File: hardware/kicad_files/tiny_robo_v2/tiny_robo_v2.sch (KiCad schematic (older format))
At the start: 31 parts, among them P1 CONN_01X06, P2 BATT, P3 CONN_01X02, P4 CONNECTOR, P5 CONNECTOR, P6 CONN_01X02, SW1 SPDT, U1 MCP73831, U2 MIC5265, U3 ESP8266-ESP-03, U4 DRV8830, U5 DRV8830

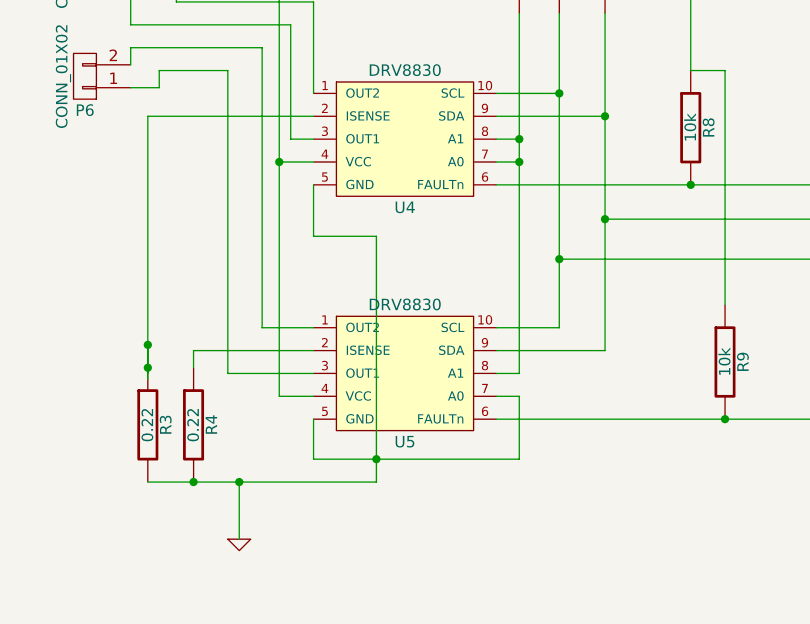
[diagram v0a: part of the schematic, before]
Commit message: syncing home version
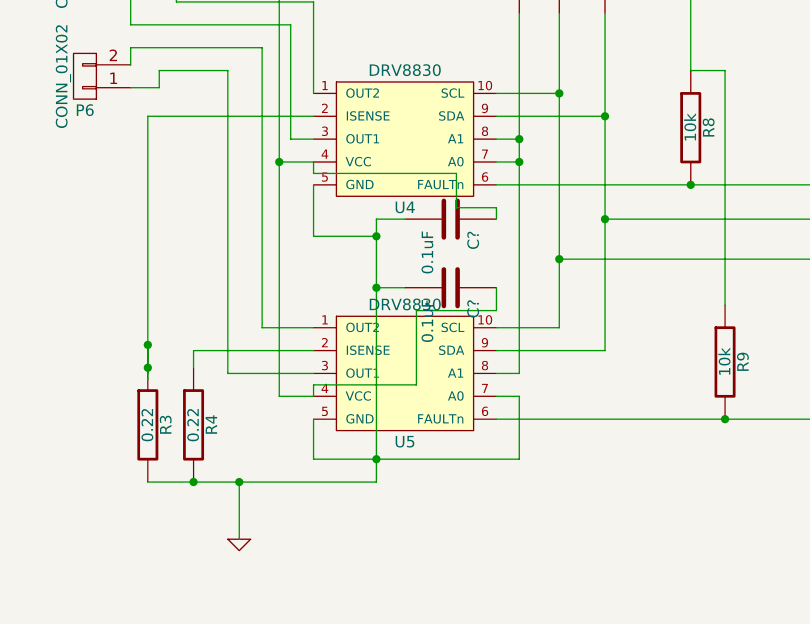
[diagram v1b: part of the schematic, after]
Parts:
- added C? (x2): 0.1uF, Capacitors_SMD:C_0805_HandSoldering, symbol C-RESCUE-tiny_robo_v2
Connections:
- net GND: now also C?.2, C?.2
- net Unreg: now also C?.1, C?.1
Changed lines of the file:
@@
 EESchema Schematic File Version 2
+LIBS:tiny_robo_v2-rescue
 LIBS:power
 LIBS:device
@@
 	5650 1300 6275 1300
 Wire Wire Line
-	8650 5525 8650 6600
+	8650 5450 8650 6600
 Connection ~ 7850 6600
 Connection ~ 9650 3775
@@
 Wire Wire Line
 	2975 4125 2400 4125
+$Comp
+L C-RESCUE-tiny_robo_v2 C?
+U 1 1 57E440DA
+P 8975 5450
+F 0 "C?" H 9025 5550 50  0000 L CNN
+F 1 "0.1uF" H 9025 5350 50  0000 L CNN
+F 2 "Capacitors_SMD:C_0805_HandSoldering" H 8975 5450 60  0001 C CNN
+F 3 "" H 8975 5450 60  0001 C CNN
+	1    8975 5450
+	0    1    1    0
+$EndComp
+$Comp
+L C-RESCUE-tiny_robo_v2 C?
+U 1 1 57E442F8
+P 8975 5750
+F 0 "C?" H 9025 5850 50  0000 L CNN
+F 1 "0.1uF" H 9025 5650 50  0000 L CNN
+F 2 "Capacitors_SMD:C_0805_HandSoldering" H 8975 5750 60  0001 C CNN
+F 3 "" H 8975 5750 60  0001 C CNN
+	1    8975 5750
+	0    1    1    0
+$EndComp
+Wire Wire Line
+	8775 5450 8650 5450
+Connection ~ 8650 5525
+Wire Wire Line
+	8775 5750 8650 5750
+Connection ~ 8650 5750
+Wire Wire Line
+	8375 6225 8375 6175
+Wire Wire Line
+	8375 6175 8825 6175
+Wire Wire Line
+	8825 6175 8825 5850
+Wire Wire Line
+	8825 5850 9175 5850
+Wire Wire Line
+	9175 5850 9175 5750
+Wire Wire Line
+	8375 5200 8375 5250
+Wire Wire Line
+	8375 5250 9000 5250
+Wire Wire Line
+	9000 5250 9000 5400
+Wire Wire Line
+	9000 5400 9175 5400
+Wire Wire Line
+	9175 5400 9175 5450
 $EndSCHEMATC
